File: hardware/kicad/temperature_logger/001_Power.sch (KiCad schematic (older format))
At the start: 22 parts, among them J2 Power, J3 USB_B_Micro, Q1 Q_PMOS_GSD, U4 AMS1117-3.3, U5 FT231XS

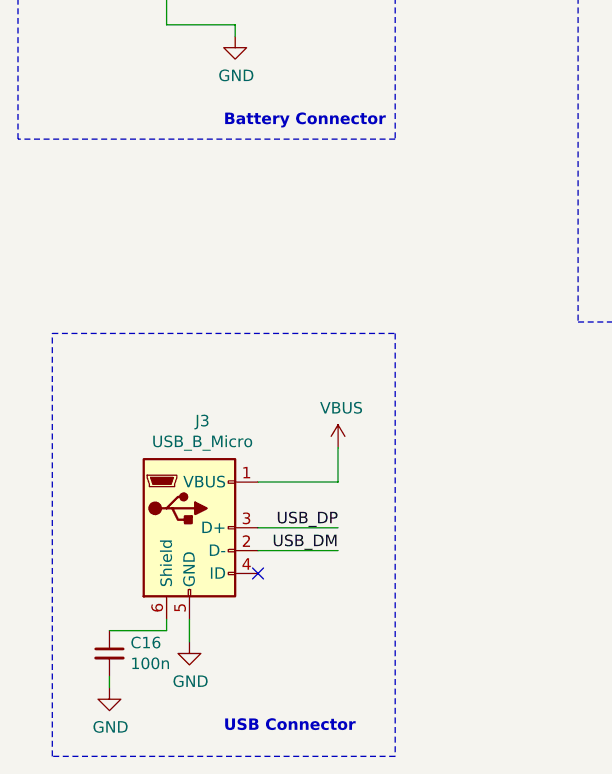
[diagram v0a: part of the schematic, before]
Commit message: Added schematic changes
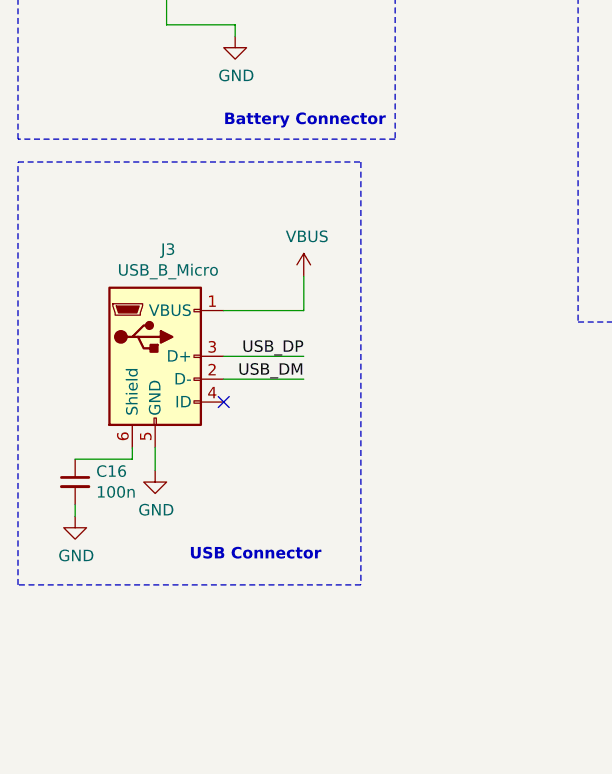
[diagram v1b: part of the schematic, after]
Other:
- moved on the sheet: C16, J3
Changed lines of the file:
@@
 encoding utf-8
 Sheet 2 2
-Title ""
-Date ""
-Rev ""
-Comp ""
+Title "Temperature Logger"
+Date "2021-09-12"
+Rev "1"
+Comp "PradS"
 Comment1 ""
 Comment2 ""
@@
 L Connector:USB_B_Micro J3
 U 1 1 60C8255D
-P 1600 4000
-F 0 "J3" H 1657 4467 50  0000 C CNN
-F 1 "USB_B_Micro" H 1657 4376 50  0000 C CNN
-F 2 "Connector_USB:USB_Micro-B_Molex-105017-0001" H 1750 3950 50  0001 C CNN
-F 3 "~" H 1750 3950 50  0001 C CNN
-	1    1600 4000
-	1    0    0    -1
-$EndComp
-Wire Wire Line
-	2250 3650 2250 3800
+P 1450 3250
+F 0 "J3" H 1507 3717 50  0000 C CNN
+F 1 "USB_B_Micro" H 1507 3626 50  0000 C CNN
+F 2 "Connector_USB:USB_Micro-B_Molex-105017-0001" H 1600 3200 50  0001 C CNN
+F 3 "~" H 1600 3200 50  0001 C CNN
+	1    1450 3250
+	1    0    0    -1
+$EndComp
+Wire Wire Line
+	2100 2900 2100 3050
 $Comp
 L power:GND #PWR?
 U 1 1 60C86ACE
-P 1600 4500
+P 1450 3750
 AR Path="/60C86ACE" Ref="#PWR?"  Part="1"
 AR Path="/60D5E44C/60C86ACE" Ref="#PWR023"  Part="1"
-F 0 "#PWR023" H 1600 4250 50  0001 C CNN
-F 1 "GND" H 1605 4327 50  0000 C CNN
-F 2 "" H 1600 4500 50  0001 C CNN
-F 3 "" H 1600 4500 50  0001 C CNN
-	1    1600 4500
-	1    0    0    -1
-$EndComp
-Wire Wire Line
-	1600 4500 1600 4400
-Text Label 2250 4100 2    50   ~ 0
+F 0 "#PWR023" H 1450 3500 50  0001 C CNN
+F 1 "GND" H 1455 3577 50  0000 C CNN
+F 2 "" H 1450 3750 50  0001 C CNN
+F 3 "" H 1450 3750 50  0001 C CNN
+	1    1450 3750
+	1    0    0    -1
+$EndComp
+Wire Wire Line
+	1450 3750 1450 3650
+Text Label 2100 3350 2    50   ~ 0
 USB_DM
-Text Label 2250 4000 2    50   ~ 0
+Text Label 2100 3250 2    50   ~ 0
 USB_DP
 Wire Wire Line
-	1900 4000 2250 4000
-Wire Wire Line
-	1900 4100 2250 4100
+	1750 3250 2100 3250
+Wire Wire Line
+	1750 3350 2100 3350
 $Comp
 L Device:R_Small R?
@@
 L power:VBUS #PWR026
 U 1 1 60C9C23F
-P 2250 3650
-F 0 "#PWR026" H 2250 3500 50  0001 C CNN
-F 1 "VBUS" H 2265 3823 50  0000 C CNN
-F 2 "" H 2250 3650 50  0001 C CNN
-F 3 "" H 2250 3650 50  0001 C CNN
-	1    2250 3650
+P 2100 2900
+F 0 "#PWR026" H 2100 2750 50  0001 C CNN
+F 1 "VBUS" H 2115 3073 50  0000 C CNN
+F 2 "" H 2100 2900 50  0001 C CNN
+F 3 "" H 2100 2900 50  0001 C CNN
+	1    2100 2900
 	1    0    0    -1
 $EndComp
@@
 $EndComp
 Wire Notes Line
-	1000 3150 2500 3150
-Wire Notes Line
-	2500 3150 2500 5000
-Wire Notes Line
-	2500 5000 1000 5000
-Wire Notes Line
-	1000 5000 1000 3150
-Text Notes 1750 4900 0    50   ~ 10
+	850  2400 2350 2400
+Wire Notes Line
+	2350 2400 2350 4250
+Wire Notes Line
+	2350 4250 850  4250
+Wire Notes Line
+	850  4250 850  2400
+Text Notes 1600 4150 0    50   ~ 10
 USB Connector
 Wire Wire Line
@@
 	1650 1350 1500 1350
 Wire Wire Line
-	1900 3800 2250 3800
-NoConn ~ 1900 4200
+	1750 3050 2100 3050
+NoConn ~ 1750 3450
 $Comp
 L Device:C_Small C?
 U 1 1 60E38EEA
-P 1250 4550
+P 1100 3800
 AR Path="/60E38EEA" Ref="C?"  Part="1"
 AR Path="/60D5E44C/60E38EEA" Ref="C16"  Part="1"
-F 0 "C16" H 1342 4596 50  0000 L CNN
-F 1 "100n" H 1342 4505 50  0000 L CNN
-F 2 "Capacitor_SMD:C_0603_1608Metric_Pad1.08x0.95mm_HandSolder" H 1250 4550 50  0001 C CNN
-F 3 "~" H 1250 4550 50  0001 C CNN
-	1    1250 4550
-	1    0    0    -1
-$EndComp
-Wire Wire Line
-	1500 4400 1500 4450
-Wire Wire Line
-	1500 4450 1250 4450
+F 0 "C16" H 1192 3846 50  0000 L CNN
+F 1 "100n" H 1192 3755 50  0000 L CNN
+F 2 "Capacitor_SMD:C_0603_1608Metric_Pad1.08x0.95mm_HandSolder" H 1100 3800 50  0001 C CNN
+F 3 "~" H 1100 3800 50  0001 C CNN
+	1    1100 3800
+	1    0    0    -1
+$EndComp
+Wire Wire Line
+	1350 3650 1350 3700
+Wire Wire Line
+	1350 3700 1100 3700
 $Comp
 L power:GND #PWR?
 U 1 1 60E3C0D0
-P 1250 4700
+P 1100 3950
 AR Path="/60E3C0D0" Ref="#PWR?"  Part="1"
 AR Path="/60D5E44C/60E3C0D0" Ref="#PWR0102"  Part="1"
-F 0 "#PWR0102" H 1250 4450 50  0001 C CNN
-F 1 "GND" H 1255 4527 50  0000 C CNN
-F 2 "" H 1250 4700 50  0001 C CNN
-F 3 "" H 1250 4700 50  0001 C CNN
-	1    1250 4700
-	1    0    0    -1
-$EndComp
-Wire Wire Line
-	1250 4650 1250 4700
+F 0 "#PWR0102" H 1100 3700 50  0001 C CNN
+F 1 "GND" H 1105 3777 50  0000 C CNN
+F 2 "" H 1100 3950 50  0001 C CNN
+F 3 "" H 1100 3950 50  0001 C CNN
+	1    1100 3950
+	1    0    0    -1
+$EndComp
+Wire Wire Line
+	1100 3900 1100 3950
 $Comp
 L power:VDC #PWR?
